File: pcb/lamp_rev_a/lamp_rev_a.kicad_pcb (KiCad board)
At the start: 4 copper layers, 100 x 80 mm, 107 parts, among them J1 TYPE-C 3.1 MT 16P, J2 DC-005-5A-2.0, J3 DB128H-5.08-2P-BK-S, Q1 AO3400A, Q2 MMBT3904, Q3 MMBT3904, Q4 MMBT3904, Q5 MMBT3904, Q6 MMBT3904, Q7 MMBT3904, Q8 MMBT3904, Q9 MMBT3904, U1 ESP32-S3-WROOM-1-N8, U2 USBLC6-2SC6, U3 AMS1117-3.3, U4 ADS1115IDGSR, U5 CD74HC4051M, U6 TLV6001IDBVR, U7 TC4427ACOA

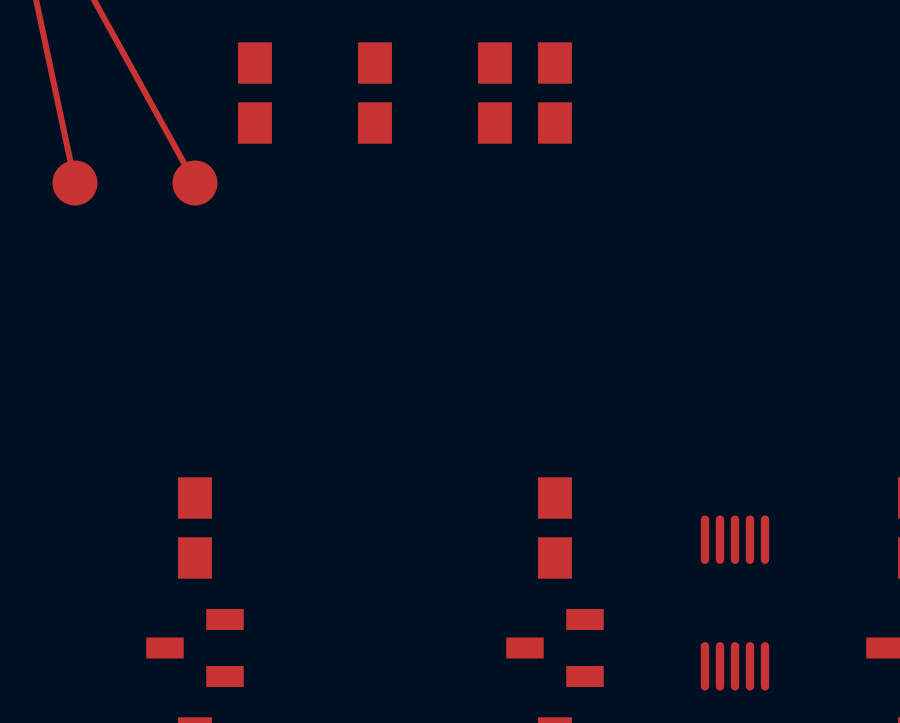
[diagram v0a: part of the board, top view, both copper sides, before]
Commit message: Tighten LAMP Rev A routing workflow
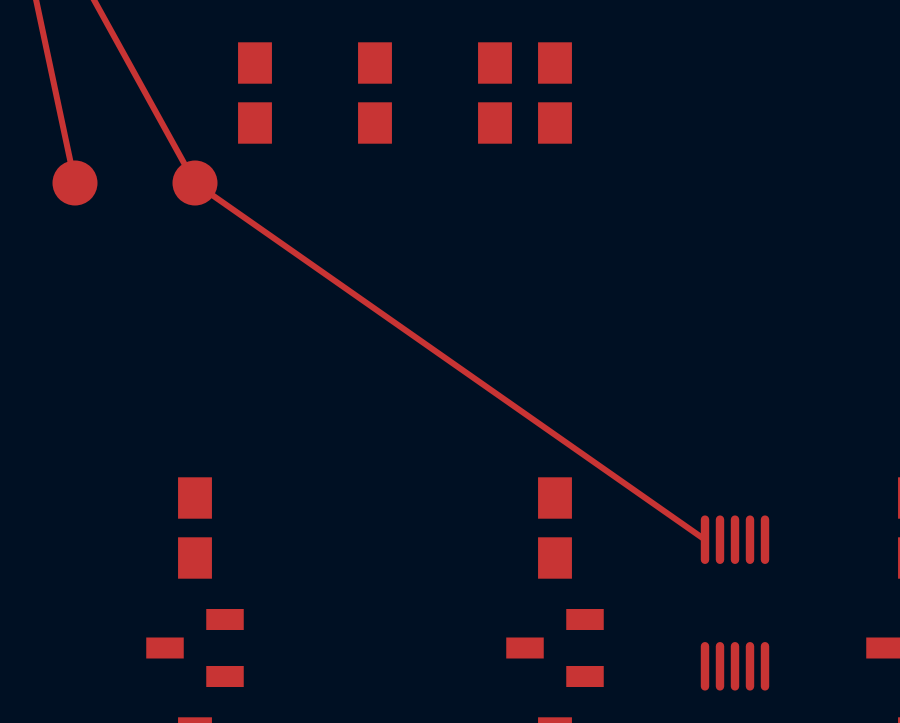
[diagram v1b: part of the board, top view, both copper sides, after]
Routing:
- net SCL: track 9.19 -> 29.9 mm
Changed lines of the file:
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@@
     (net 26)
+  )
+  (segment
+    (start 32 34)
+    (end 49 45.890)
+    (width 0.200)
+    (layer "F.Cu")
+    (net 12)
   )
   (zone
